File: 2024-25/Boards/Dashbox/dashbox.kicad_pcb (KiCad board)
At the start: 2 copper layers, 90 x 75 mm, 15 parts, among them J1 Conn_01x06_Socket, J2 Conn_01x06_Socket, J3 Conn_01x06_Socket, U1 SN65HVD230

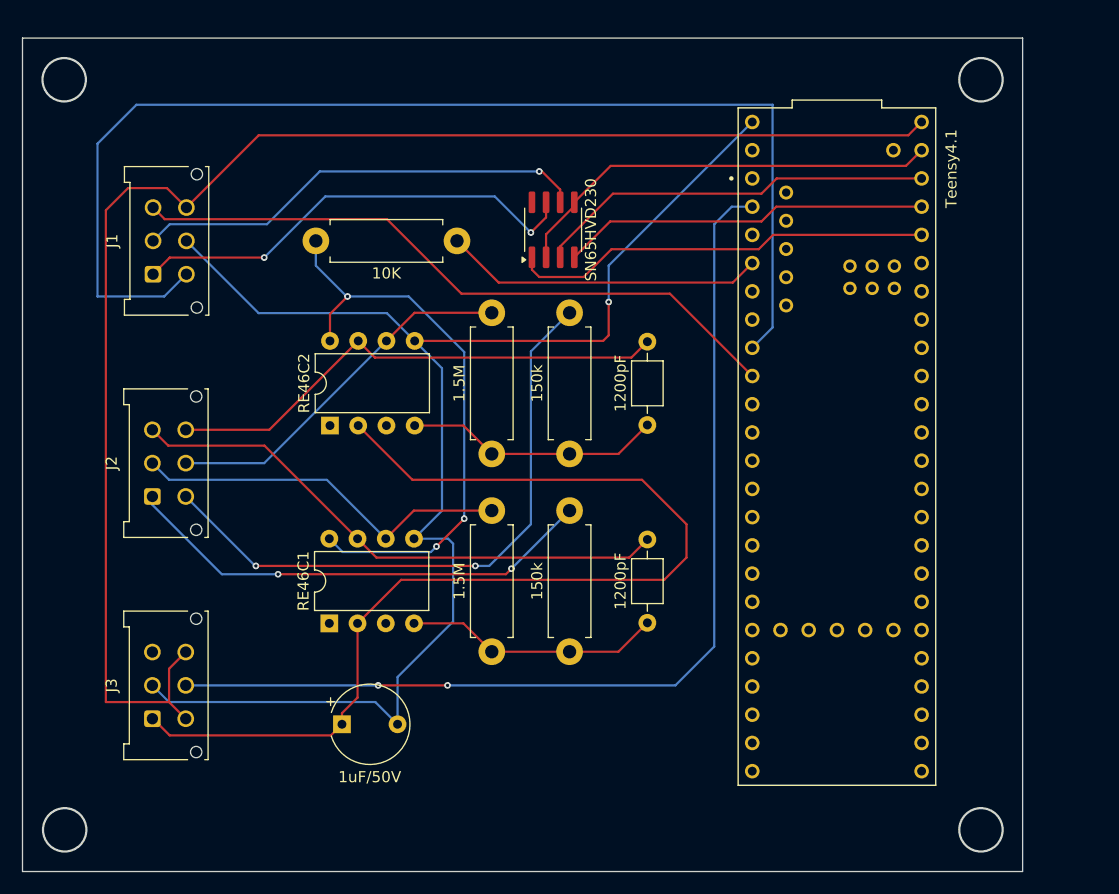
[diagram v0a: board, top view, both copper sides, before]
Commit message: dashbox pcb
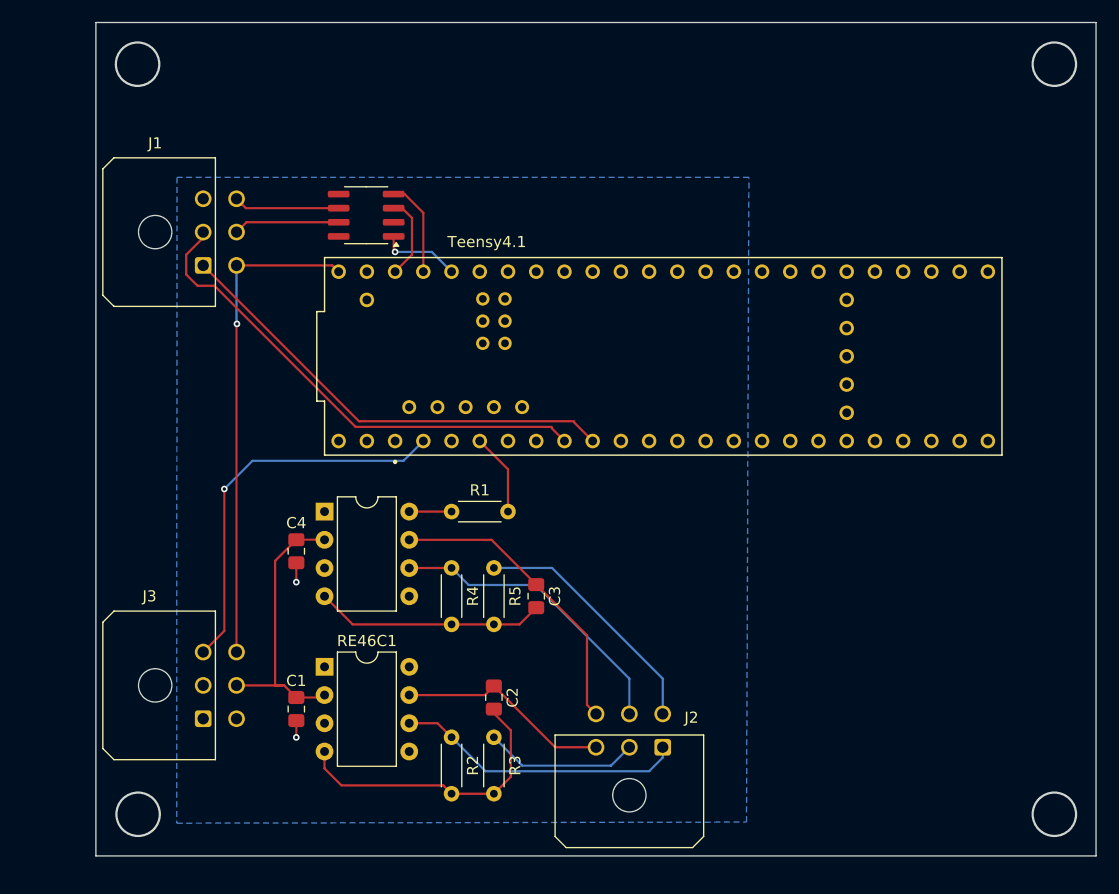
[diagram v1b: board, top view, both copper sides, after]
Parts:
- added C4: 1uF/50V, Capacitor_SMD:C_0805_2012Metric_Pad1.18x1.45mm_HandSolder, F.Cu at (135.9, 89.9)
- C1: footprint Capacitor_THT:CP_Radial_Tantal_D7.0mm_P5.00mm -> Capacitor_SMD:C_0805_2012Metric_Pad1.18x1.45mm_HandSolder
- C2, C3: footprint Capacitor_THT:C_Axial_L3.8mm_D2.6mm_P7.50mm_Horizontal -> Capacitor_SMD:C_0805_2012Metric_Pad1.18x1.45mm_HandSolder
- J1, J2, J3: value Conn_01x06_Socket -> 430450600; footprint Connector_Molex:Molex_Micro-Fit_3.0_43045-0612_2x03_P3.00mm_Vertical -> Connector_Molex:Molex_Micro-Fit_3.0_43045-0600_2x03_P3.00mm_Horizontal
- R1, R2, R3, R4, R5: footprint Resistor_THT:R_Axial_DIN0411_L9.9mm_D3.6mm_P12.70mm_Horizontal -> Resistor_THT:R_Axial_DIN0204_L3.6mm_D1.6mm_P5.08mm_Horizontal
- moved J2 51.2 mm to (168.9, 107.6), turned to 180 degrees
- moved R1 27.2 mm to (149.9, 86.4)
- moved C3 25.0 mm to (157.5, 94.0)
- moved R5 23.9 mm to (153.7, 91.4)
- moved R4 23.2 mm to (149.9, 91.4)
- moved R3 21.5 mm to (153.7, 106.7)
- moved R2 20.7 mm to (149.9, 106.7)
- moved C2 19.8 mm to (153.7, 103.1)
- moved Teensy4.1 17.6 mm to (168.9, 72.4), turned to 0 degrees
- moved U1 16.9 mm to (142.2, 59.7), turned to 180 degrees
- moved RE46C2 7.76 mm to (138.4, 86.4), turned to 0 degrees
- moved J1 4.58 mm to (127.5, 64.2)
- moved J3 4.57 mm to (127.5, 105.0)
- moved C1 4.33 mm to (135.9, 104.1), turned to -90 degrees
- moved RE46C1 3.93 mm to (138.4, 100.3), turned to 0 degrees
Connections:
- C1 pad 2: SPK_GND -> GND
- J1 pad 1: CANH -> Net-(J1-Pin_1)
- J1 pad 2: CANL -> Net-(J1-Pin_2)
- J1 pad 3: Net-(J1-Pin_3) -> GND
- J1 pad 4: Net-(J1-Pin_4) -> 5V+
- J1 pad 5: SPK_GND -> CANH
- J1 pad 6: /TNSY_5V+ -> CANL
- J2 pad 1: Speaker1_F -> Speaker1_G
- J2 pad 2: Speaker1_G -> Speaker1_F
- J3 pad 1: SPK_12V+ -> unconnected-(J3-Pin_1-Pad1)
- J3 pad 2: SPK_GND -> GND
- J3 pad 3: Reset -> R2D
- J3 pad 4: /TNSY_5V+ -> 5V+
- J3 pad 5: R2D -> SPK_12V+
- J3 pad 6: /TNSY_5V+ -> 5V+
- RE46C1 pad 5: SPK_GND -> GND
- RE46C2 pad 5: SPK_GND -> GND
- Teensy4.1 pad 7: Net-(J1-Pin_4) -> Net-(J1-Pin_2)
- Teensy4.1 pad 8: Net-(J1-Pin_3) -> Net-(J1-Pin_1)
- Teensy4.1 pad GND1: SPK_GND -> GND
- Teensy4.1 pad GND3: Net-(U1-GND) -> unconnected-(Teensy4.1-GND-PadGND3)
- Teensy4.1 pad VIN: /TNSY_5V+ -> 5V+
- U1 pad 2: Net-(U1-GND) -> unconnected-(U1-GND-Pad2)
- U1 pad 5: Net-(U1-GND) -> unconnected-(U1-Vref-Pad5)
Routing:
- net /TNSY_5V+: track 135.3 -> 0.00 mm
- net SPK_GND: track 131.9 -> 0.00 mm, vias 1 -> 0
- net Net-(J1-Pin_4): track 107.4 -> 0.00 mm
- net SPK_12V+: track 96.0 -> 25.5 mm
- net Net-(J1-Pin_3): track 60.2 -> 0.00 mm
- net R2D: track 91.1 -> 35.3 mm, vias 2 -> 1
- net Net-(RE46C1-HRNEN): track 52.3 -> 3.81 mm, vias 3 -> 0
- net Net-(J1-Pin_2): track 0.00 -> 44.8 mm
- net 5V+: track 0.00 -> 44.2 mm, vias 0 -> 1
- net Net-(J1-Pin_1): track 0.00 -> 41.5 mm
- net Net-(U1-GND): track 39.2 -> 0.00 mm
- net Speaker2_F: track 55.8 -> 22.5 mm, vias 2 -> 0
- net CANH: track 41.5 -> 9.56 mm, vias 2 -> 0
- net CANL: track 41.0 -> 9.54 mm, vias 1 -> 0
- net Net-(Teensy4.1-CTX1): track 38.0 -> 7.27 mm, vias 0 -> 1
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- added copper zone on B.Cu, net GND
